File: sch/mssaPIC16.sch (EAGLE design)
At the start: 32 parts, among them IC1 PIC16F676P, IC2 7805L, Q1 BC550C, Q2 BC550C

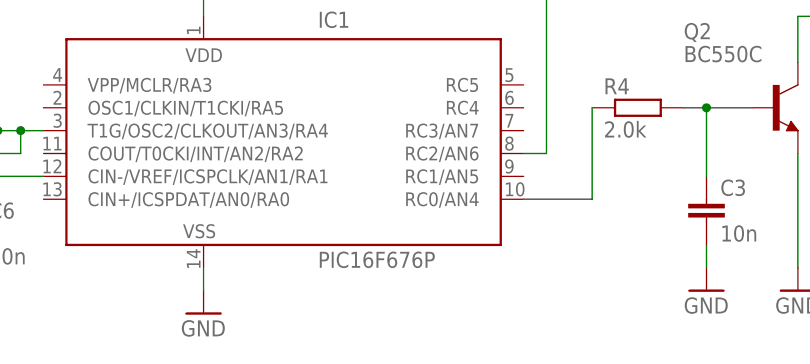
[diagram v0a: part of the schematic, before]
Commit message: Add files via upload
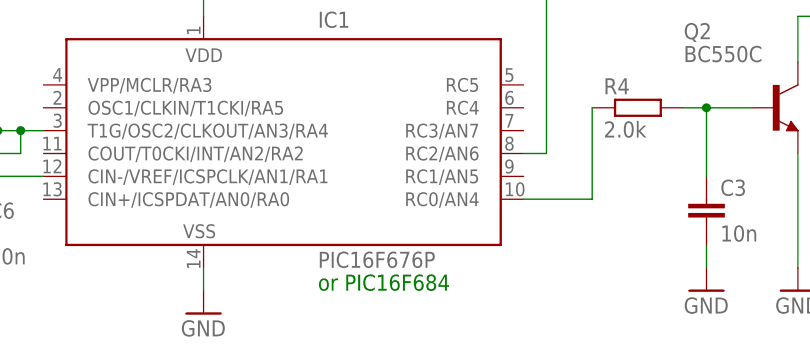
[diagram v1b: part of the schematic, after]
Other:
- note added: "or PIC16F684"
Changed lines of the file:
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@@
 <plain>
 <text x="25.4" y="109.22" size="3.81" layer="91">LZ2HV T-Cross</text>
+<text x="78.74" y="27.94" size="1.778" layer="91">or PIC16F684</text>
 </plain>
 <instances>
